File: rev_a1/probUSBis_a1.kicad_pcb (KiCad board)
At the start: 2 copper layers, 44.5 x 22.9 mm, 23 parts, among them CON1 USB-MINI-B, IC1 ATTINY85-P, P1 USB_A_MALE, P2 CONN_8, P3 CONN_4, U1 LM78L05ACZ

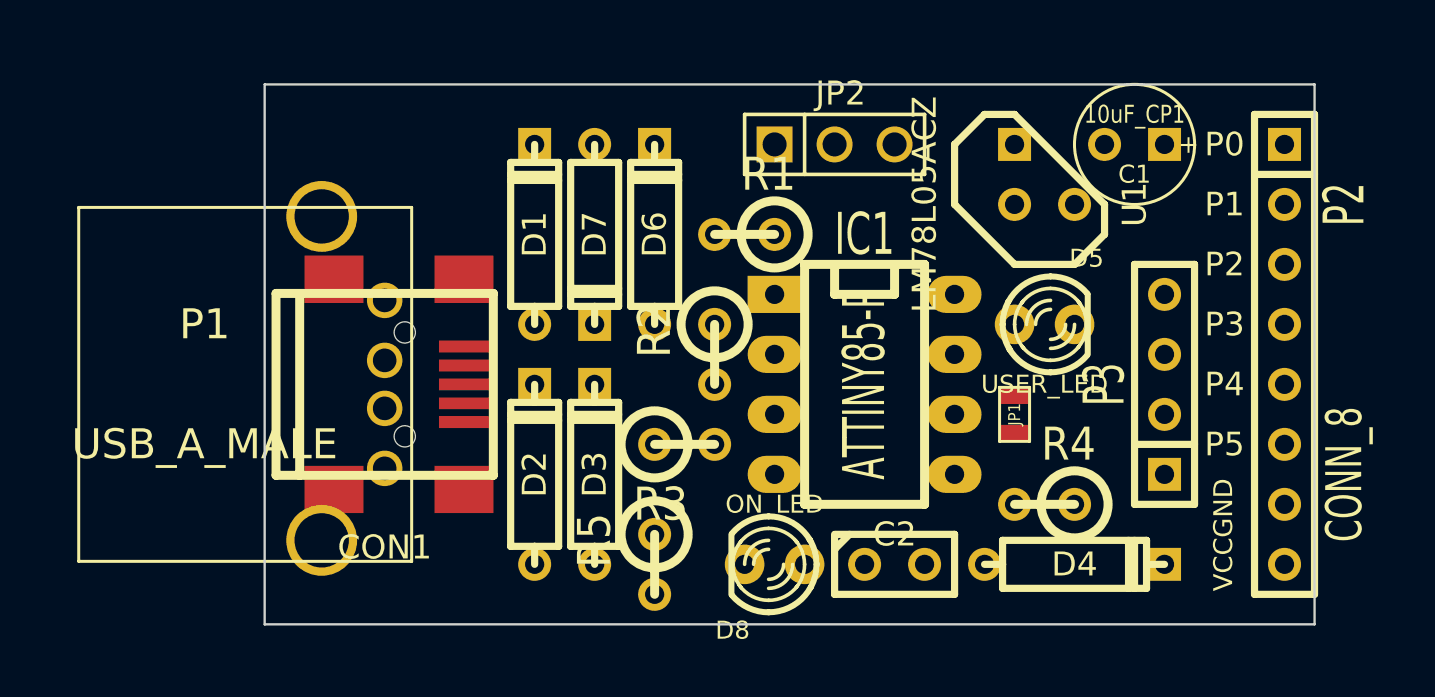
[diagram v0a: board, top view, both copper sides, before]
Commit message: editing pcb layout, trying to compress more
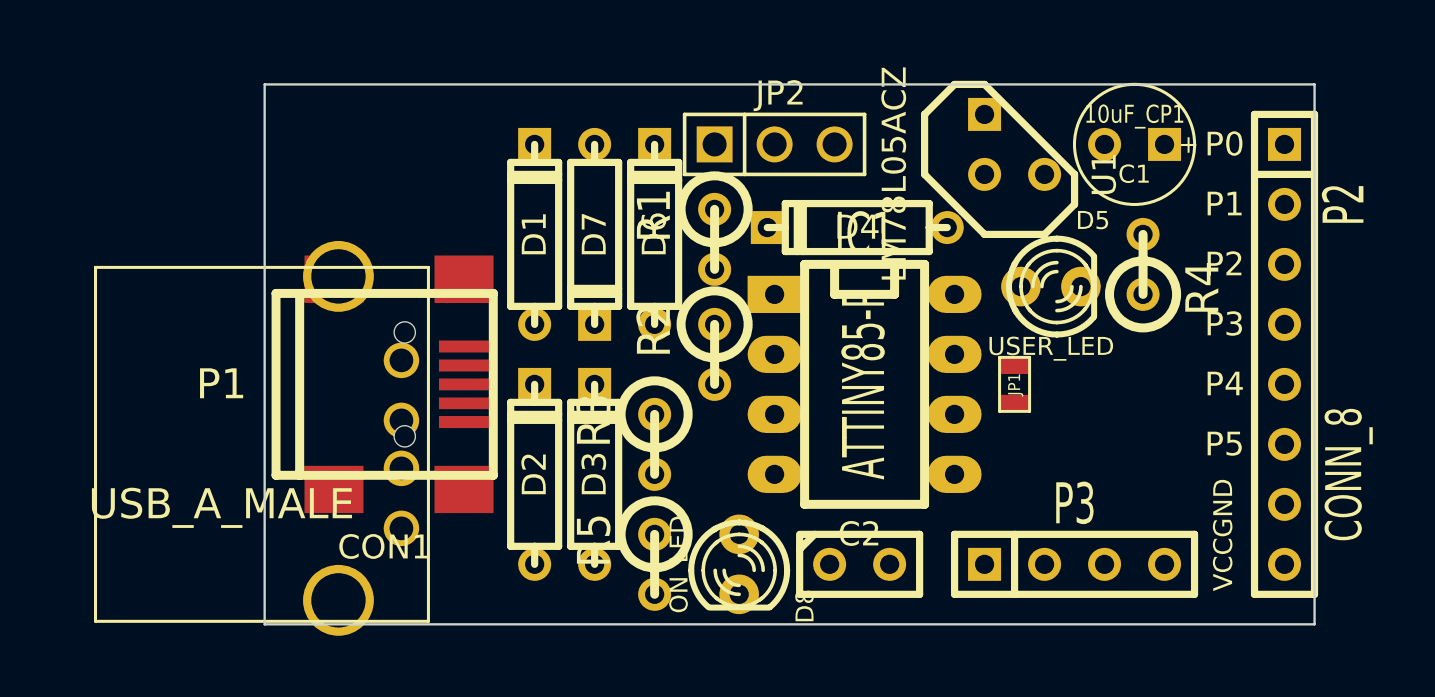
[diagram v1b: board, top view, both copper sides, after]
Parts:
- moved D4 17.0 mm to (130.5, 97.5), turned to 180 degrees
- moved R4 11.0 mm to (142.6, 99.1), turned to 90 degrees
- moved P3 8.52 mm to (139.7, 111.8), turned to 0 degrees
- moved P1 2.64 mm to (111.2, 106.7)
- moved JP2 2.54 mm to (127.0, 94.0)
- moved U1 1.80 mm to (137.2, 94.0)
- moved D5 1.62 mm to (138.7, 100.0)
- moved D8 1.50 mm to (125.5, 111.8), turned to 270 degrees
- moved C2 1.48 mm to (130.6, 111.8)
- moved R1 1.29 mm to (124.5, 98.0), turned to 270 degrees
- moved JP1 1.27 mm to (137.2, 104.1)
- moved R3 1.27 mm to (121.9, 106.7), turned to 270 degrees
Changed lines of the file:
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@@
   )
   (module C1 (layer F.Cu)
-    (at 132.08 111.76)
+    (at 130.6 111.76)
     (descr "Condensateur e = 1 pas")
     (tags C)
@@
   )
   (module D3 (layer F.Cu)
-    (at 139.7 111.76)
+    (at 130.5 97.5 180)
     (descr "Diode 3 pas")
     (tags "DIODE DEV")
-    (fp_text reference D4 (at 0 0) (layer F.SilkS)
-      (effects (font (size 1.016 1.016) (thickness 0.2032)))
-    )
-    (fp_text value DIODE (at 0 0) (layer F.SilkS) hide
+    (fp_text reference D4 (at 0 0 180) (layer F.SilkS)
+      (effects (font (size 1.016 1.016) (thickness 0.2032)))
+    )
+    (fp_text value DIODE (at 0 0 180) (layer F.SilkS) hide
       (effects (font (size 1.016 1.016) (thickness 0.2032)))
     )
@@
     (fp_line (start 2.54 -1.016) (end 2.54 1.016) (layer F.SilkS) (width 0.3048))
     (fp_line (start 2.286 1.016) (end 2.286 -1.016) (layer F.SilkS) (width 0.3048))
-    (pad 2 thru_hole rect (at 3.81 0) (size 1.397 1.397) (drill 0.8128)
+    (pad 2 thru_hole rect (at 3.81 0 180) (size 1.397 1.397) (drill 0.8128)
       (layers *.Cu *.Mask F.SilkS)
       (net 2 +5V)
     )
-    (pad 1 thru_hole circle (at -3.81 0) (size 1.397 1.397) (drill 0.8128)
+    (pad 1 thru_hole circle (at -3.81 0 180) (size 1.397 1.397) (drill 0.8128)
       (layers *.Cu *.Mask F.SilkS)
       (net 8 N-0000016)
@@
   )
   (module LED-3MM (layer F.Cu)
-    (at 138.43 101.6)
+    (at 138.7 100)
     (descr "LED 3mm - Lead pitch 100mil (2,54mm)")
     (tags "LED led 3mm 3MM 100mil 2,54mm")
@@
   )
   (module LED-3MM (layer F.Cu)
-    (at 127 111.76 180)
+    (at 125.5 111.76 270)
     (descr "LED 3mm - Lead pitch 100mil (2,54mm)")
     (tags "LED led 3mm 3MM 100mil 2,54mm")
-    (fp_text reference D8 (at 1.778 -2.794 180) (layer F.SilkS)
+    (fp_text reference D8 (at 1.778 -2.794 270) (layer F.SilkS)
       (effects (font (size 0.762 0.762) (thickness 0.0889)))
     )
-    (fp_text value ON_LED (at 0 2.54 180) (layer F.SilkS)
+    (fp_text value ON_LED (at 0 2.54 270) (layer F.SilkS)
       (effects (font (size 0.762 0.762) (thickness 0.0889)))
     )
@@
     (fp_arc (start 0.254 0) (end -1.778 0) (angle 28.3) (layer F.SilkS) (width 0.254))
     (fp_arc (start 0.254 0) (end -1.47574 1.06426) (angle 31.6) (layer F.SilkS) (width 0.254))
-    (pad 1 thru_hole circle (at -1.27 0 180) (size 1.6764 1.6764) (drill 0.8128)
+    (pad 1 thru_hole circle (at -1.27 0 270) (size 1.6764 1.6764) (drill 0.8128)
       (layers *.Cu *.Mask F.SilkS)
       (net 19 VCC)
     )
-    (pad 2 thru_hole circle (at 1.27 0 180) (size 1.6764 1.6764) (drill 0.8128)
+    (pad 2 thru_hole circle (at 1.27 0 270) (size 1.6764 1.6764) (drill 0.8128)
       (layers *.Cu *.Mask F.SilkS)
       (net 18 N-000009)
@@
   )
   (module PIN_ARRAY_3X1 (layer F.Cu)
-    (at 129.54 93.98)
+    (at 127 93.98)
     (descr "Connecteur 3 pins")
     (tags "CONN DEV")
@@
   )
   (module USB_A (layer F.Cu)
-    (at 110.49 104.14 180)
+    (at 111.2 106.68 180)
     (fp_text reference P1 (at 7.62 2.54 180) (layer F.SilkS)
       (effects (font (thickness 0.3048)))
@@
   )
   (module SIL-4 (layer F.Cu)
-    (at 143.51 104.14 90)
+    (at 139.7 111.76)
     (descr "Connecteur 4 pibs")
     (tags "CONN DEV")
-    (fp_text reference P3 (at 0 -2.54 90) (layer F.SilkS)
+    (fp_text reference P3 (at 0 -2.54) (layer F.SilkS)
       (effects (font (size 1.73482 1.08712) (thickness 0.3048)))
     )
-    (fp_text value CONN_4 (at 0 -2.54 90) (layer F.SilkS) hide
+    (fp_text value CONN_4 (at 0 -2.54) (layer F.SilkS) hide
       (effects (font (size 1.524 1.016) (thickness 0.3048)))
     )
@@
     (fp_line (start 5.08 1.27) (end -5.08 1.27) (layer F.SilkS) (width 0.3048))
     (fp_line (start -2.54 1.27) (end -2.54 -1.27) (layer F.SilkS) (width 0.3048))
-    (pad 1 thru_hole rect (at -3.81 0 90) (size 1.397 1.397) (drill 0.8128)
+    (pad 1 thru_hole rect (at -3.81 0) (size 1.397 1.397) (drill 0.8128)
       (layers *.Cu *.Mask F.SilkS)
       (net 1 +3.3V)
     )
-    (pad 2 thru_hole circle (at -1.27 0 90) (size 1.397 1.397) (drill 0.8128)
+    (pad 2 thru_hole circle (at -1.27 0) (size 1.397 1.397) (drill 0.8128)
       (layers *.Cu *.Mask F.SilkS)
       (net 2 +5V)
     )
-    (pad 3 thru_hole circle (at 1.27 0 90) (size 1.397 1.397) (drill 0.8128)
-      (layers *.Cu *.Mask F.SilkS)
-      (net 3 GND)
-    )
-    (pad 4 thru_hole circle (at 3.81 0 90) (size 1.397 1.397) (drill 0.8128)
+    (pad 3 thru_hole circle (at 1.27 0) (size 1.397 1.397) (drill 0.8128)
+      (layers *.Cu *.Mask F.SilkS)
+      (net 3 GND)
+    )
+    (pad 4 thru_hole circle (at 3.81 0) (size 1.397 1.397) (drill 0.8128)
       (layers *.Cu *.Mask F.SilkS)
       (net 20 VIN)
@@
   )
   (module R1 (layer F.Cu)
-    (at 125.73 97.79 180)
+    (at 124.46 98 270)
     (descr "Resistance verticale")
     (tags R)
     (autoplace_cost90 10)
     (autoplace_cost180 10)
-    (fp_text reference R1 (at -1.016 2.54 180) (layer F.SilkS)
-      (effects (font (size 1.397 1.27) (thickness 0.2032)))
-    )
-    (fp_text value 1.5K_R (at -1.143 2.54 180) (layer F.SilkS) hide
+    (fp_text reference R1 (at -1.016 2.54 270) (layer F.SilkS)
+      (effects (font (size 1.397 1.27) (thickness 0.2032)))
+    )
+    (fp_text value 1.5K_R (at -1.143 2.54 270) (layer F.SilkS) hide
       (effects (font (size 1.397 1.27) (thickness 0.2032)))
     )
     (fp_line (start -1.27 0) (end 1.27 0) (layer F.SilkS) (width 0.381))
     (fp_circle (center -1.27 0) (end -0.635 1.27) (layer F.SilkS) (width 0.381))
-    (pad 1 thru_hole circle (at -1.27 0 180) (size 1.397 1.397) (drill 0.8128)
+    (pad 1 thru_hole circle (at -1.27 0 270) (size 1.397 1.397) (drill 0.8128)
       (layers *.Cu *.Mask F.SilkS)
       (net 19 VCC)
     )
-    (pad 2 thru_hole circle (at 1.27 0 180) (size 1.397 1.397) (drill 0.8128)
+    (pad 2 thru_hole circle (at 1.27 0 270) (size 1.397 1.397) (drill 0.8128)
       (layers *.Cu *.Mask F.SilkS)
       (net 11 N-0000019)
@@
   )
   (module R1 (layer F.Cu)
-    (at 123.19 106.68)
+    (at 121.92 106.68 270)
     (descr "Resistance verticale")
     (tags R)
     (autoplace_cost90 10)
     (autoplace_cost180 10)
-    (fp_text reference R3 (at -1.016 2.54) (layer F.SilkS)
-      (effects (font (size 1.397 1.27) (thickness 0.2032)))
-    )
-    (fp_text value 68R (at -1.143 2.54) (layer F.SilkS) hide
+    (fp_text reference R3 (at -1.016 2.54 270) (layer F.SilkS)
+      (effects (font (size 1.397 1.27) (thickness 0.2032)))
+    )
+    (fp_text value 68R (at -1.143 2.54 270) (layer F.SilkS) hide
       (effects (font (size 1.397 1.27) (thickness 0.2032)))
     )
     (fp_line (start -1.27 0) (end 1.27 0) (layer F.SilkS) (width 0.381))
     (fp_circle (center -1.27 0) (end -0.635 1.27) (layer F.SilkS) (width 0.381))
-    (pad 1 thru_hole circle (at -1.27 0) (size 1.397 1.397) (drill 0.8128)
+    (pad 1 thru_hole circle (at -1.27 0 270) (size 1.397 1.397) (drill 0.8128)
       (layers *.Cu *.Mask F.SilkS)
       (net 9 N-0000017)
     )
-    (pad 2 thru_hole circle (at 1.27 0) (size 1.397 1.397) (drill 0.8128)
+    (pad 2 thru_hole circle (at 1.27 0 270) (size 1.397 1.397) (drill 0.8128)
       (layers *.Cu *.Mask F.SilkS)
       (net 7 N-0000015)
@@
   )
   (module R1 (layer F.Cu)
-    (at 138.43 109.22 180)
+    (at 142.6 99.06 90)
     (descr "Resistance verticale")
     (tags R)
     (autoplace_cost90 10)
     (autoplace_cost180 10)
-    (fp_text reference R4 (at -1.016 2.54 180) (layer F.SilkS)
-      (effects (font (size 1.397 1.27) (thickness 0.2032)))
-    )
-    (fp_text value 1K_R (at -1.143 2.54 180) (layer F.SilkS) hide
+    (fp_text reference R4 (at -1.016 2.54 90) (layer F.SilkS)
+      (effects (font (size 1.397 1.27) (thickness 0.2032)))
+    )
+    (fp_text value 1K_R (at -1.143 2.54 90) (layer F.SilkS) hide
       (effects (font (size 1.397 1.27) (thickness 0.2032)))
     )
     (fp_line (start -1.27 0) (end 1.27 0) (layer F.SilkS) (width 0.381))
     (fp_circle (center -1.27 0) (end -0.635 1.27) (layer F.SilkS) (width 0.381))
-    (pad 1 thru_hole circle (at -1.27 0 180) (size 1.397 1.397) (drill 0.8128)
+    (pad 1 thru_hole circle (at -1.27 0 90) (size 1.397 1.397) (drill 0.8128)
       (layers *.Cu *.Mask F.SilkS)
       (net 5 N-0000011)
     )
-    (pad 2 thru_hole circle (at 1.27 0 180) (size 1.397 1.397) (drill 0.8128)
+    (pad 2 thru_hole circle (at 1.27 0 90) (size 1.397 1.397) (drill 0.8128)
       (layers *.Cu *.Mask F.SilkS)
       (net 3 GND)
@@
   )
   (module TO92-123 (layer F.Cu)
-    (at 138.43 95.25 90)
+    (at 137.16 93.98 90)
     (descr "Transistor TO92 brochage type BC237")
     (tags "TR TO92")
@@
   )
   (module SM0603 (layer F.Cu)
-    (at 137.16 105.41 90)
+    (at 137.16 104.14 90)
     (attr smd)
     (fp_text reference JP1 (at 0 0 90) (layer F.SilkS)
